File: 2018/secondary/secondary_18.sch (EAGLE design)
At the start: 9 parts

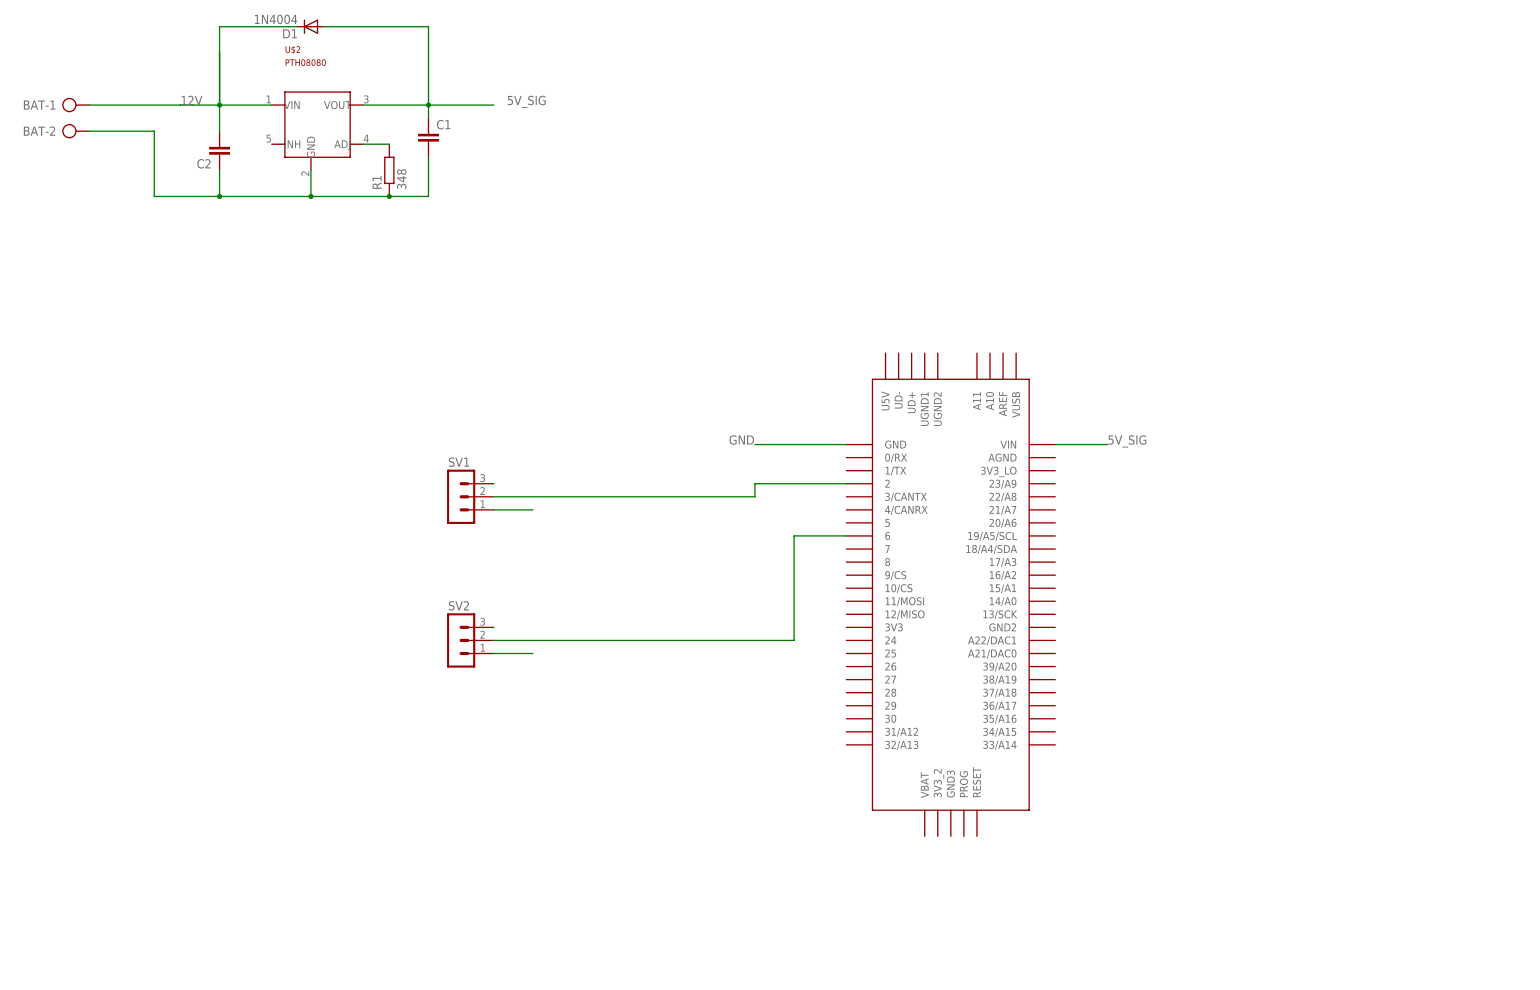
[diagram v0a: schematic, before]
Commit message: [Secondary] Finishes the 2018 schematic
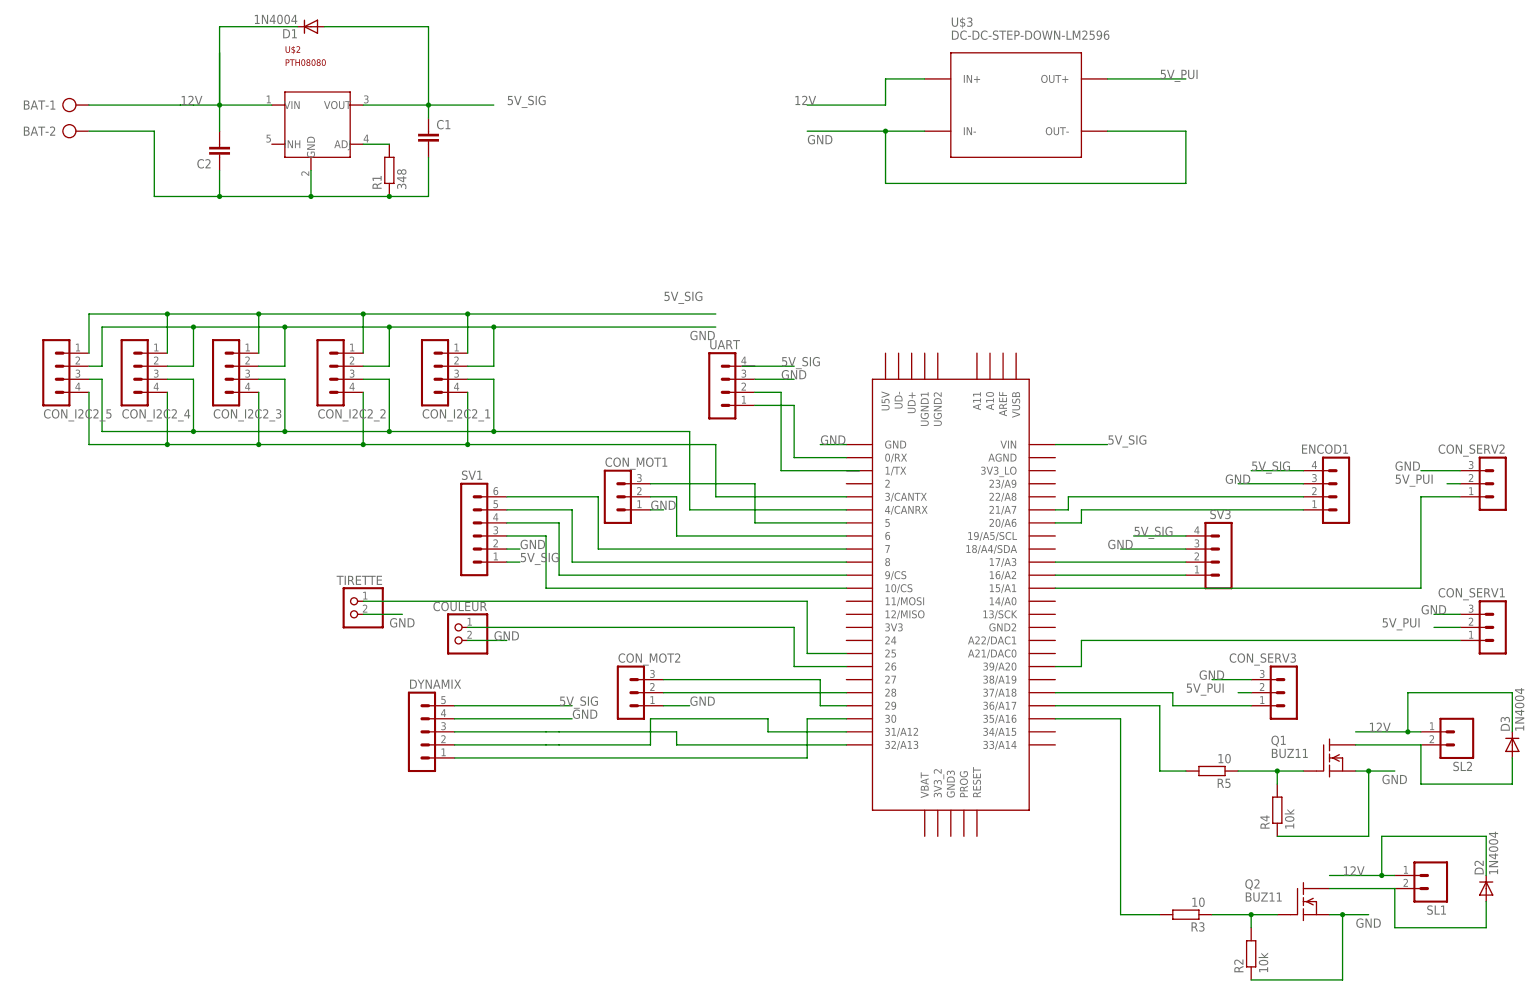
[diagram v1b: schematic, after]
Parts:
- removed SV2: (no value), con-lstb:MA03-1
- added CON_I2C2_1, CON_I2C2_2, CON_I2C2_3, CON_I2C2_4, CON_I2C2_5, ENCOD1, SV3, UART: (no value), con-lstb:MA04-1
- added CON_MOT1, CON_MOT2, CON_SERV1, CON_SERV2, CON_SERV3: (no value), con-lstb:MA03-1
- added COULEUR, TIRETTE: (no value), pinhead:PINHD-1X2
- added D2, D3: 1N4004, diode:1N4004
- added DYNAMIX: (no value), con-lstb:MA05-1
- added Q1, Q2: BUZ11, transistor-fet:BUZ11
- added R2, R4: 10k, resistor:R-EU_0204/7
- added R3, R5: 10, resistor:R-EU_0204/7
- added SL1, SL2: (no value), con-amp-quick:MA02
- added U$3: DC-DC-STEP-DOWN-LM2596, diy-modules:DC-DC-STEP-DOWN-LM2596
- SV1: device con-lstb:MA03-1 -> con-lstb:MA06-1
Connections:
- new net 5V_PUI: CON_SERV1.2, CON_SERV2.2, CON_SERV3.2, U$3.OUT+
- new net N$10: Q1.G, R4.2, R5.1
- new net N$11: R5.2, U$1.36/A17
- new net N$12: D3.A, Q1.D, SL2.2
- new net N$13: SV3.2, U$1.17/A3
- new net N$14: ENCOD1.1, U$1.20/A6
- new net N$15: ENCOD1.2, U$1.21/A7
- new net N$16: CON_SERV2.1, U$1.15/A1
- new net N$17: CON_SERV3.1, U$1.37/A18
- new net N$18: DYNAMIX.3, U$1.32/A13
- new net N$19: CON_SERV1.1, U$1.39/A20
- new net N$2: CON_MOT2.3, U$1.29
- new net N$20: DYNAMIX.2, U$1.31/A12
- new net N$21: CON_I2C2_1.4, CON_I2C2_2.4, CON_I2C2_3.4, CON_I2C2_4.4, CON_I2C2_5.4, U$1.3/CANTX
- new net N$22: COULEUR.1, U$1.26
- new net N$23: CON_I2C2_1.3, CON_I2C2_2.3, CON_I2C2_3.3, CON_I2C2_4.3, CON_I2C2_5.3, U$1.4/CANRX
- new net N$24: DYNAMIX.1, U$1.30
- new net N$25: TIRETTE.1, U$1.25
- new net N$26: UART.2
- new net N$27: U$1.0/RX, UART.1
- new net N$3: CON_MOT1.3, U$1.5
- new net N$30: SV1.3, U$1.10/CS
- new net N$31: SV1.4, U$1.9/CS
- new net N$32: SV1.5, U$1.8
- new net N$33: SV1.6, U$1.7
- new net N$6: Q2.G, R2.2, R3.1
- new net N$7: R3.2, U$1.35/A16
- new net N$8: D2.A, Q2.D, SL1.2
- new net N$9: SV3.1, U$1.16/A2
- net 12V: now also D2.C, D3.C, SL1.1, SL2.1, U$3.IN+
- net 5V_SIG: now also CON_I2C2_1.1, CON_I2C2_2.1, CON_I2C2_3.1, CON_I2C2_4.1, CON_I2C2_5.1, DYNAMIX.5, ENCOD1.4, SV1.1, SV3.4
- net GND: now also CON_I2C2_1.2, CON_I2C2_2.2, CON_I2C2_3.2, CON_I2C2_4.2, CON_I2C2_5.2, CON_MOT1.1, CON_MOT2.1, CON_SERV1.3, CON_SERV2.3, CON_SERV3.3, COULEUR.2, DYNAMIX.4, ENCOD1.3, Q1.S, Q2.S, R2.1, R4.1, SV1.2, SV3.3, TIRETTE.2, U$3.IN-, U$3.OUT-, UART.3; no longer SV1.1, SV2.1
- net N$4: now also CON_MOT1.2, U$1.6; no longer SV1.2, U$1.2
- net N$5: now also CON_MOT2.2, U$1.28; no longer SV2.2, U$1.6
